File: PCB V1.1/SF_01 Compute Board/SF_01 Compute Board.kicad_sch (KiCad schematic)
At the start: 25 parts, among them J1 SS-53200-001, J15 USB_C_Receptacle_USB2.0_16P, Q1 BSS138, SW1 POWER, SW2 PI_BOOT, SW6 SW_DPDT_x2, U1 CM4102008, U2 TPD4E02B04DQA, U3 TPD4E02B04DQA, U7 TPD4E02B04DQA, U8 74LVC1G07, U9 74LVC1G07

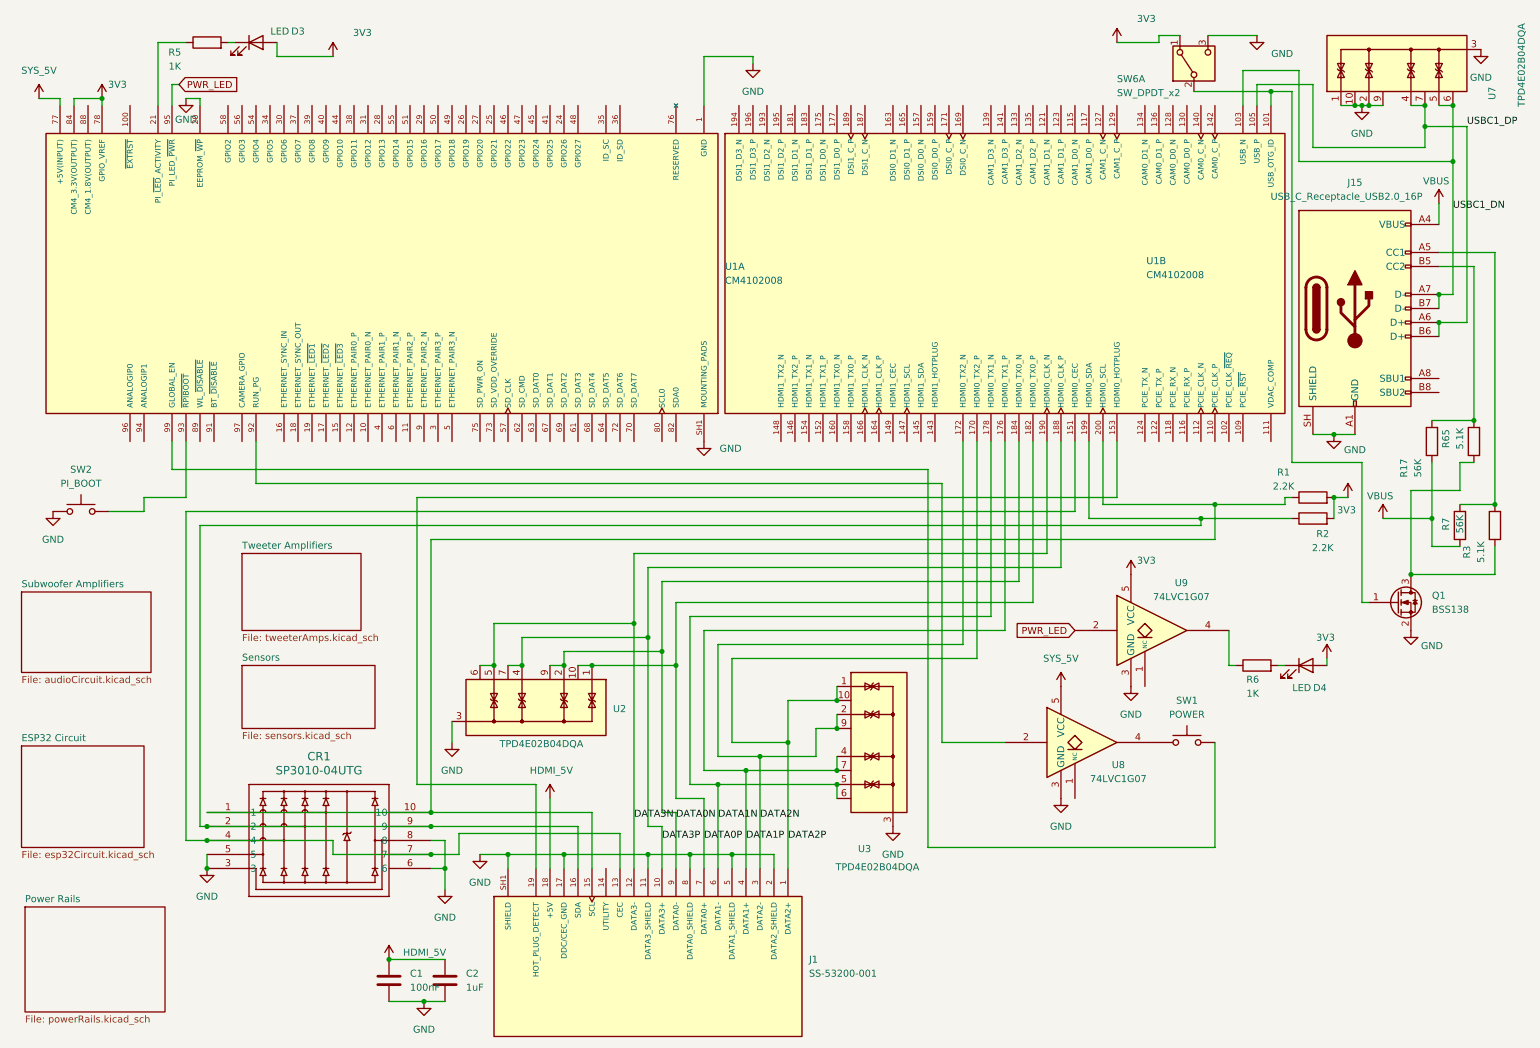
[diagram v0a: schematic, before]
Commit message: Finished final version of PCB and BOM
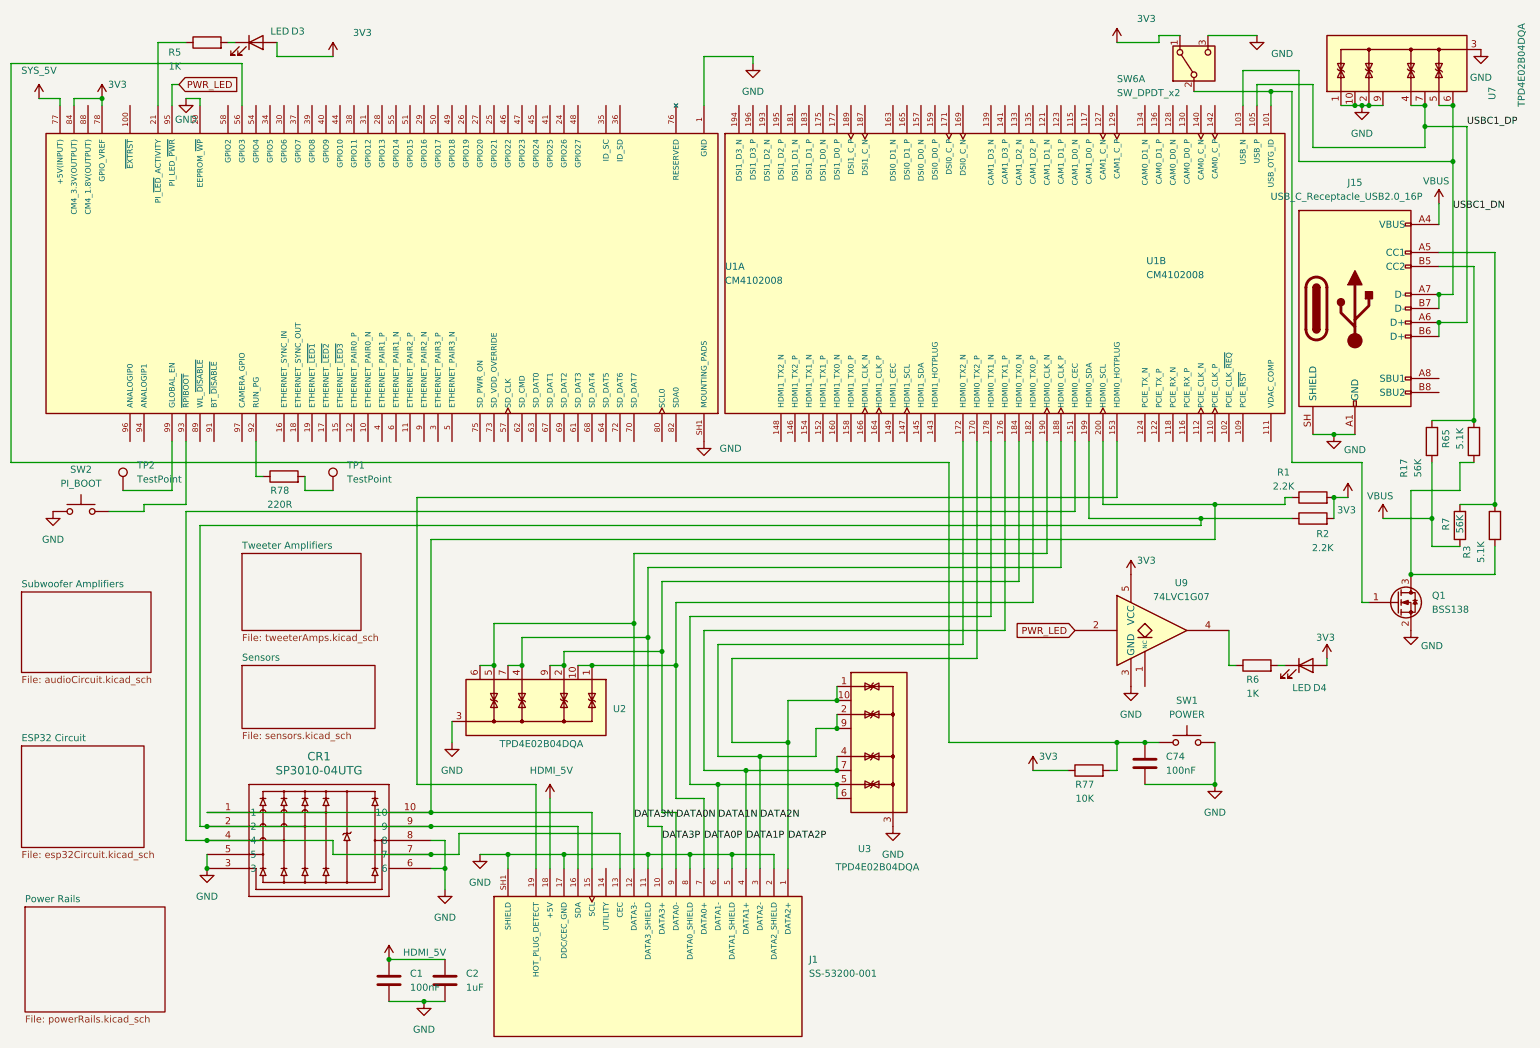
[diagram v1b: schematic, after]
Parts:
- removed U8: 74LVC1G07, Package_TO_SOT_SMD:SOT-23-5, symbol 74xGxx:74LVC1G07
- added C74: 100nF, Capacitor_SMD:C_0603_1608Metric, symbol Device:C
- added R77: 10K, Resistor_SMD:R_0603_1608Metric, symbol Device:R
- added R78: 220R, Resistor_SMD:R_0603_1608Metric, symbol Device:R
- added TP1, TP2: TestPoint, TestPoint:TestPoint_Pad_3.0x3.0mm, symbol Connector:TestPoint
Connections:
- net 3V3: now also R77.1
- net GND: now also SW1.2, C74.2
- net at SW1.1: now also U1.56 (GPIO3), C74.1, R77.2
- net at U1.99 (GLOBAL_EN): now also TP2.1; no longer SW1.2
- net at U1.92 (RUN_PG): now also R78.1
- new net: R78.2, TP1.1
